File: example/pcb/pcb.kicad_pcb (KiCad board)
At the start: 2 copper layers, 9.8 x 16.4 mm, 7 parts, among them IC1 DS4432U+T&R, J1 Conn_01x06_Pin

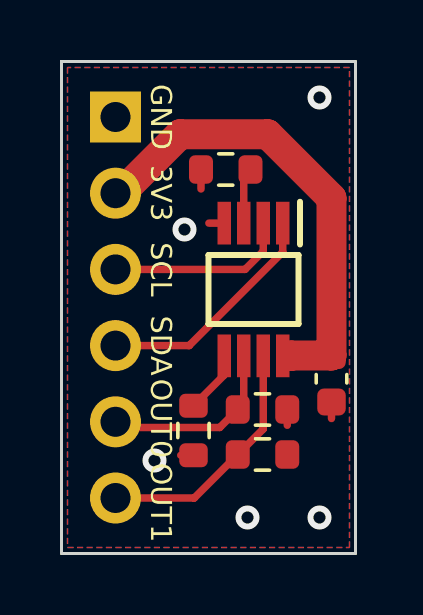
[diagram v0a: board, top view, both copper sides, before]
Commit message: Update pcb
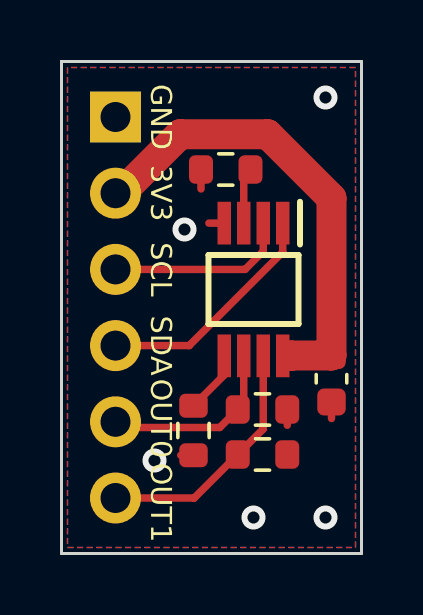
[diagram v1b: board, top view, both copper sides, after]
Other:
- board size 9.8 x 16.4 mm -> 10 x 16.4 mm
- board text added: "JLCJLCJLCJLC"
